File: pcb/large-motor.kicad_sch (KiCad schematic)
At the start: 1 part, among them U1 ACS781xLRTR-100B

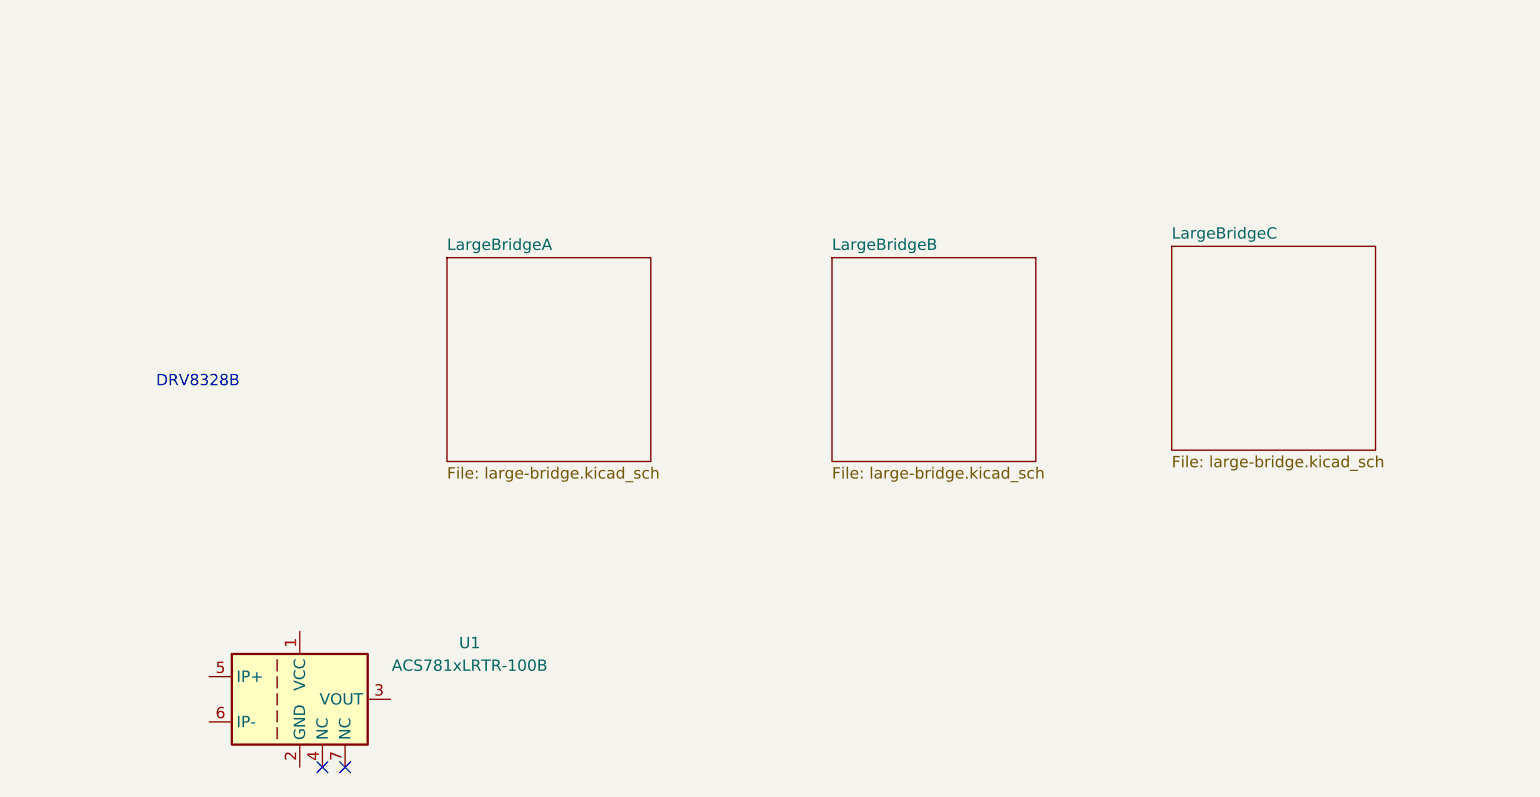
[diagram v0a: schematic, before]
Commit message: Save progress
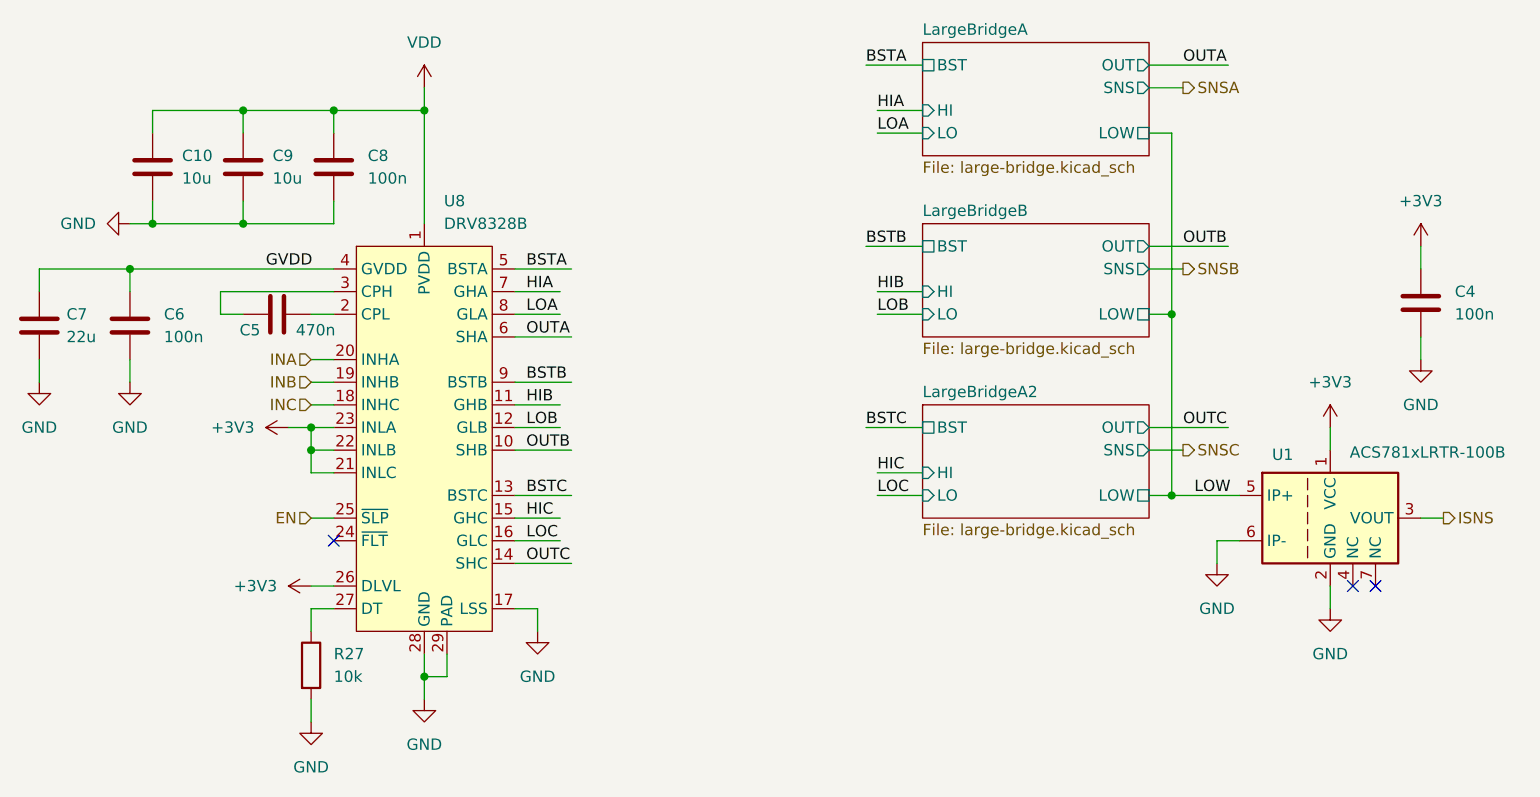
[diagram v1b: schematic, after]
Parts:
- added C10, C9: 10u, Capacitor_SMD:C_0805_2012Metric, symbol Device:C
- added C4, C6, C8: 100n, Capacitor_SMD:C_0402_1005Metric, symbol Device:C
- added C5: 470n, Capacitor_SMD:C_0603_1608Metric, symbol Device:C
- added C7: 22u, Capacitor_SMD:C_0805_2012Metric, symbol Device:C
- added R27: 10k, Resistor_SMD:R_0402_1005Metric, symbol Device:R
- added U8: DRV8328B, Package_DFN_QFN:QFN-28-1EP_4x4mm_P0.4mm_EP2.6x2.6mm, symbol User_Symbols:DRV8328B
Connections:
- net +3V3: now reaches U1.1 (VCC)
- net +3V3: now also C4.1, U8.21 (INLC), U8.22 (INLB), U8.23 (INLA), U8.26 (DLVL)
- net GND: now reaches U1.2 (GND)
- net GND: now also U1.6 (IP-), C10.2, C4.2, C6.2, C7.2, C8.2, C9.2, R27.2, U8.17 (LSS), U8.28 (GND), U8.29 (PAD)
- net ISNS: now reaches U1.3 (VOUT)
- net LOW: now reaches U1.5 (IP+)
- new net: R27.1, U8.27 (DT)
- new net: C5.1, U8.2 (CPL)
- new net: C5.2, U8.3 (CPH)
- new net BSTA: U8.5 (BSTA)
- new net BSTB: U8.9 (BSTB)
- new net BSTC: U8.13 (BSTC)
- new net EN: U8.25 (~{SLP})
- new net GVDD: C6.1, C7.1, U8.4 (GVDD)
- new net HIA: U8.7 (GHA)
- new net HIB: U8.11 (GHB)
- new net HIC: U8.15 (GHC)
- new net INA: U8.20 (INHA)
- new net INB: U8.19 (INHB)
- new net INC: U8.18 (INHC)
- new net LOA: U8.8 (GLA)
- new net LOB: U8.12 (GLB)
- new net LOC: U8.16 (GLC)
- new net OUTA: U8.6 (SHA)
- new net OUTB: U8.10 (SHB)
- new net OUTC: U8.14 (SHC)
- new net VDD: C10.1, C8.1, C9.1, U8.1 (PVDD)
- no-connect marks 2 -> 3
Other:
- removed sheet LargeBridgeC
- added sheet LargeBridgeA2 (large-bridge.kicad_sch)
- sheet LargeBridgeA ports: added BST, HI, LO, LOW, OUT, SNS; removed none
- sheet LargeBridgeB ports: added BST, HI, LO, LOW, OUT, SNS; removed none
- note removed: "DRV8328B"
- moved on the sheet: U1
